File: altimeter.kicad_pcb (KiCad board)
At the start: 2 copper layers, 27.9 x 15.2 mm, 16 parts, among them J1 Conn_01x03_Male, J2 Conn_01x05_Male, J3 Conn_01x05_Male, U1 TLV760, U2 test, U4 RN4871, U6 BMP280

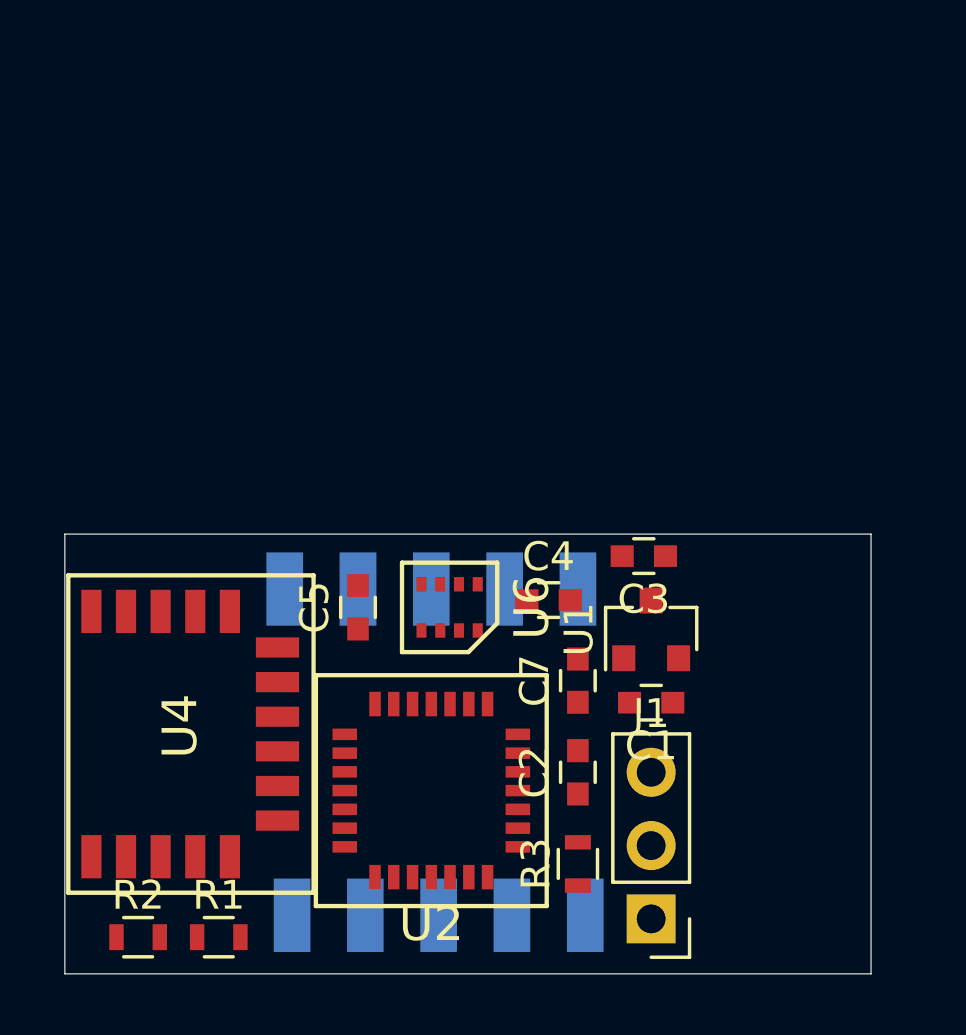
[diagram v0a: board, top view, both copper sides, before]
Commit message: wip
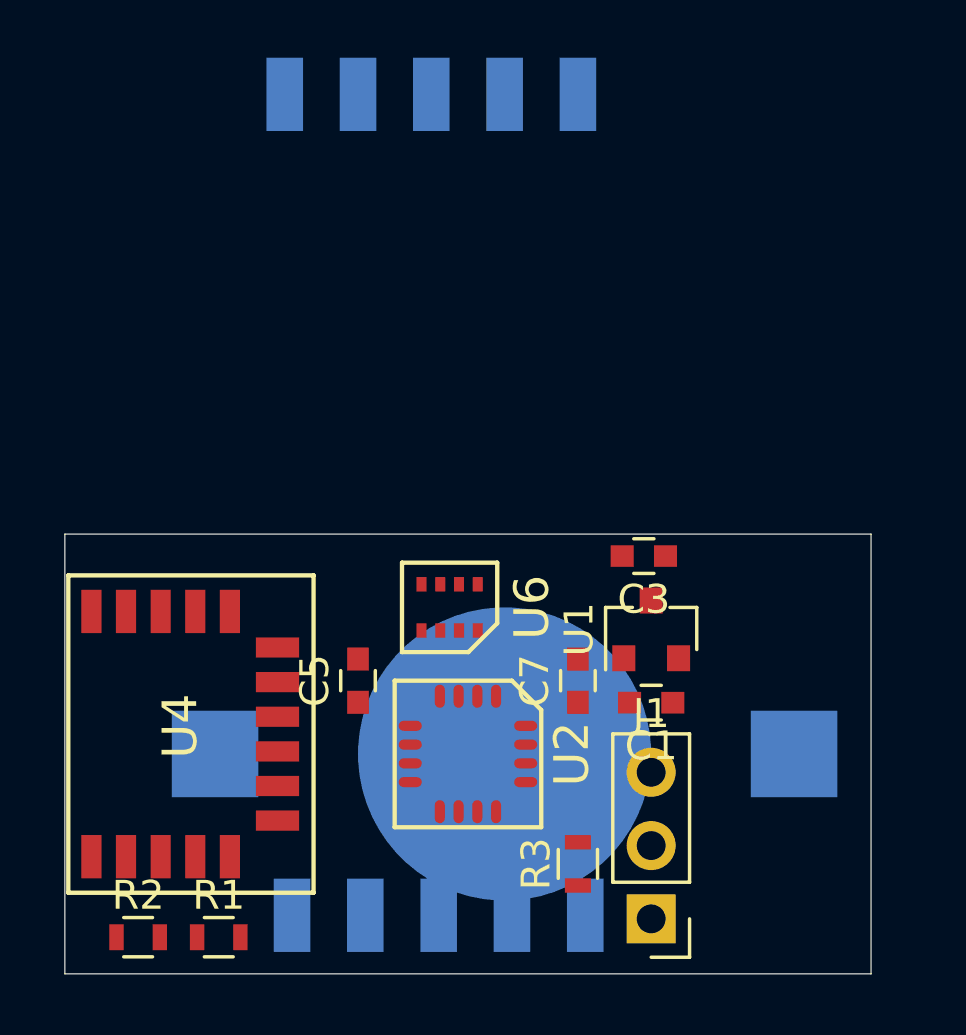
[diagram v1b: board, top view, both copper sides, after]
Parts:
- removed C2: 0.1u, Capacitors_SMD:C_0603
- removed C4: 10u, Capacitors_SMD:C_0603
- added B1: 1632-holder, lib:1632-holder, B.Cu at (78.7, 55.9)
- U2: value test -> PIC16F15325; footprint lib:QFN_28 -> lib:UQFN_16
- moved J3 17.1 mm to (76.2, 33.0)
- moved C5 2.54 mm to (73.7, 53.3)
- moved U2 1.80 mm to (77.5, 55.9), turned to 270 degrees
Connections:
- U2 pad 10: +3V3 -> Net-(U2-Pad10)
- U2 pad 11: DEBUG -> PGC
- U2 pad 12: Net-(U2-Pad12) -> PGD
- U2 pad 13: SCK -> VSS
- U2 pad 14: SDO -> (no net)
- U2 pad 15: SDI -> (no net)
- U2 pad 16: VSS -> +3V3
- U2 pad 2: (no net) -> Net-(R1-Pad1)
- U2 pad 3: PGC -> MCLR
- U2 pad 4: PGD -> DEBUG
- U2 pad 5: VSS -> U1TX
- U2 pad 6: (no net) -> U1RX
- U2 pad 7: (no net) -> SDO
- U2 pad 8: (no net) -> SDI
- U2 pad 9: (no net) -> SCK
- U6 pad 2: Net-(U2-Pad12) -> Net-(U2-Pad10)

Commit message: DEV1 basic
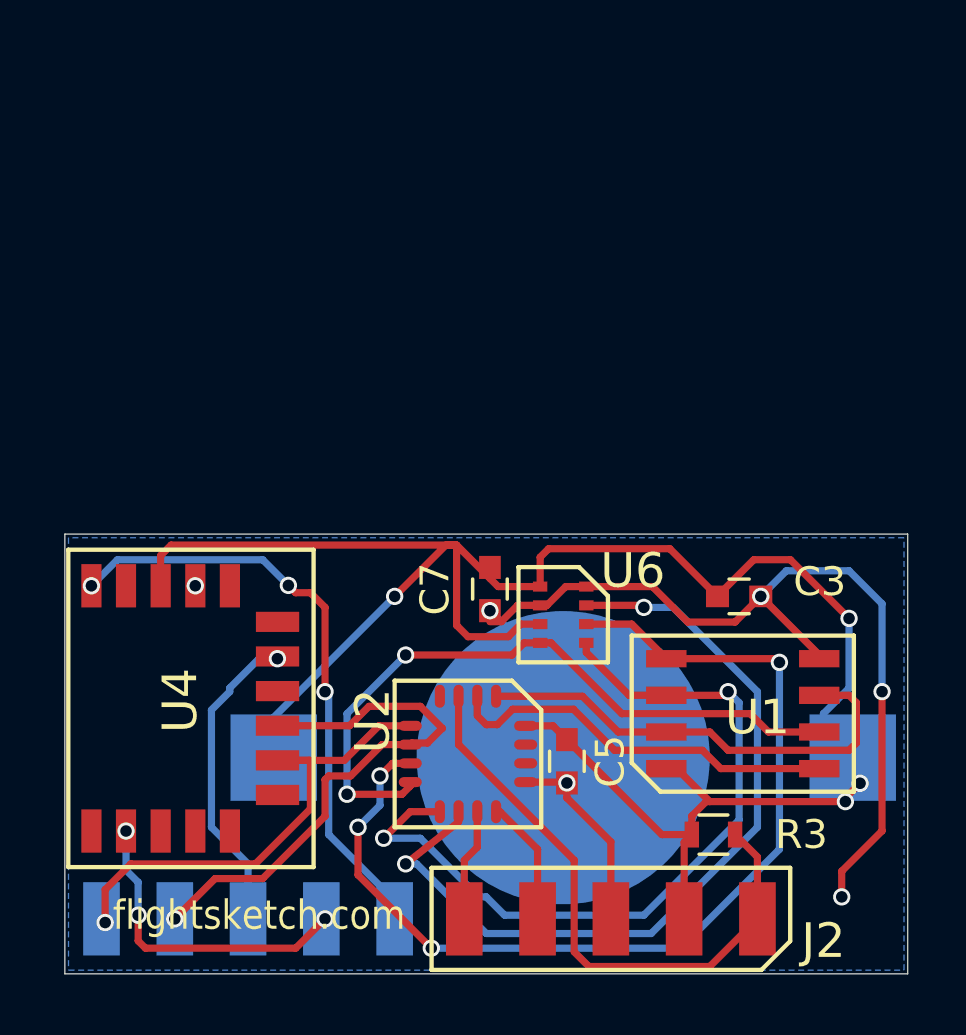
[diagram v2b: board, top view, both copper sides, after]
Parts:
- removed C1: 10u, Capacitors_SMD:C_0603
- removed J1: Conn_01x03_Male, Pin_Headers:Pin_Header_Straight_1x03_Pitch2.54mm
- removed R1: 200k, Resistors_SMD:R_0603
- removed R2: 100k, Resistors_SMD:R_0603
- J2: moved to F.Cu
- U1: value TLV760 -> EEPROM; footprint TO_SOT_Packages_SMD:SOT-23 -> lib:SO8
- moved J3 29.3 mm to (69.8, 61.6)
- moved C5 7.76 mm to (80.9, 56.1), turned to 270 degrees
- moved J2 5.97 mm to (82.4, 61.6), turned to 180 degrees
- moved R3 4.81 mm to (86.0, 58.7), turned to 180 degrees
- moved C7 4.40 mm to (78.2, 50.2), turned to 270 degrees
- moved U1 4.31 mm to (87.0, 54.5)
- moved U6 3.95 mm to (80.8, 51.1), turned to 270 degrees
- moved C3 3.59 mm to (86.9, 50.4), turned to 0 degrees
- moved B1 2.04 mm to (80.8, 56.0)
- moved U4 0.89 mm to (71.1, 58.8)
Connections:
- B1 pad 2: +3V3 -> VIN
- C3 pad 1: +3V3 -> VIN
- C5 pad 1: +3V3 -> VIN
- C7 pad 1: +3V3 -> VIN
- J2 pad 2: +3V3 -> VIN
- R3 pad 2: +3V3 -> VIN
- U1 pad 1: +3V3 -> EEPROM_CS
- U1 pad 2: VIN -> SDI
- U1 pad 3: VSS -> EEPROM_HOLD
- U2 pad 1: (no net) -> EEPROM_HOLD
- U2 pad 16: +3V3 -> VIN
- U2 pad 2: Net-(R1-Pad1) -> EEPROM_CS
- U2 pad 4: DEBUG -> (no net)
- U4 pad 14: +3V3 -> VIN
- U6 pad 6: +3V3 -> VIN
- U6 pad 8: +3V3 -> VIN
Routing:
- net VIN: track 0.00 -> 73.3 mm, vias 0 -> 4
- net VSS: track 0.00 -> 54.6 mm, vias 0 -> 9
- net SDO: track 0.00 -> 35.8 mm, vias 0 -> 4
- net Net-(U2-Pad10): track 0.00 -> 29.3 mm, vias 0 -> 2
- net SCK: track 0.00 -> 27.6 mm, vias 0 -> 2
- net SDI: track 0.00 -> 23.9 mm, vias 0 -> 2
- net MCLR: track 0.00 -> 21.0 mm
- net Net-(J3-Pad1): track 0.00 -> 20.9 mm, vias 0 -> 3
- net U1RX: track 0.00 -> 19.1 mm, vias 0 -> 1
- net U1TX: track 0.00 -> 17.5 mm, vias 0 -> 1
- net EEPROM_HOLD: track 0.00 -> 16.2 mm
- net EEPROM_CS: track 0.00 -> 13.7 mm
- net Net-(J3-Pad3): track 0.00 -> 12.3 mm, vias 0 -> 1
- net PGD: track 0.00 -> 4.39 mm
- net PGC: track 0.00 -> 3.90 mm
- added copper zone on B.Cu, net VSS
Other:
- board size 27.9 x 15.2 mm -> 29.2 x 15.2 mm
- board text added: "Basic - DEV1 vSK01.00"
- board text added: "flightsketch.com"
- board text removed: "Flight Sketch DEV2 vSK01.00 2018-04-28 Russ Parrish"
